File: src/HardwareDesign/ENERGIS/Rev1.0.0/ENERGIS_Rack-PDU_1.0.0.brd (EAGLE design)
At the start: 210 x 108 mm, 395 parts, among them IC1 MP2315GJ-Z, IC10 HLW8032, IC11 HLW8032, IC12 HLW8032, IC13 MP150GJ, IC14 HLW8032, IC15 RP2040, IC16 HLW8032, IC17 MCP6001R, IC18 W25Q128JVPIQ, IC19 CAT24C512HU5IGT3, IC2 MP2315S, IC20 W5500, IC21 MIC5504-3.3YM5-TR, IC22 MCP6001R, IC3 ULN2803A, IC4 MCP23017-E/ML, IC5 MP150GJ, IC6 HLW8032, IC7 HLW8032, IC8 HLW8032, IC9 SN74HC151PWR, J10 0R, J2 JP, J7 JP, J8 0R, J9 0R, K1 G2RL-1A-E_DC12, K2 G2RL-1A-E_DC12, K3 G2RL-1A-E_DC12, K4 G2RL-1A-E_DC12, K5 G2RL-1A-E_DC12, K6 G2RL-1A-E_DC12, K7 G2RL-1A-E_DC12, K8 G2RL-1A-E_DC12, P12ON LEDC1608X35N_FLAT-G, P3ON LEDC1608X35N_FLAT-G, P5ON LEDC1608X35N_FLAT-G, SW3 TP, X1 12MHz, X2 25MHz

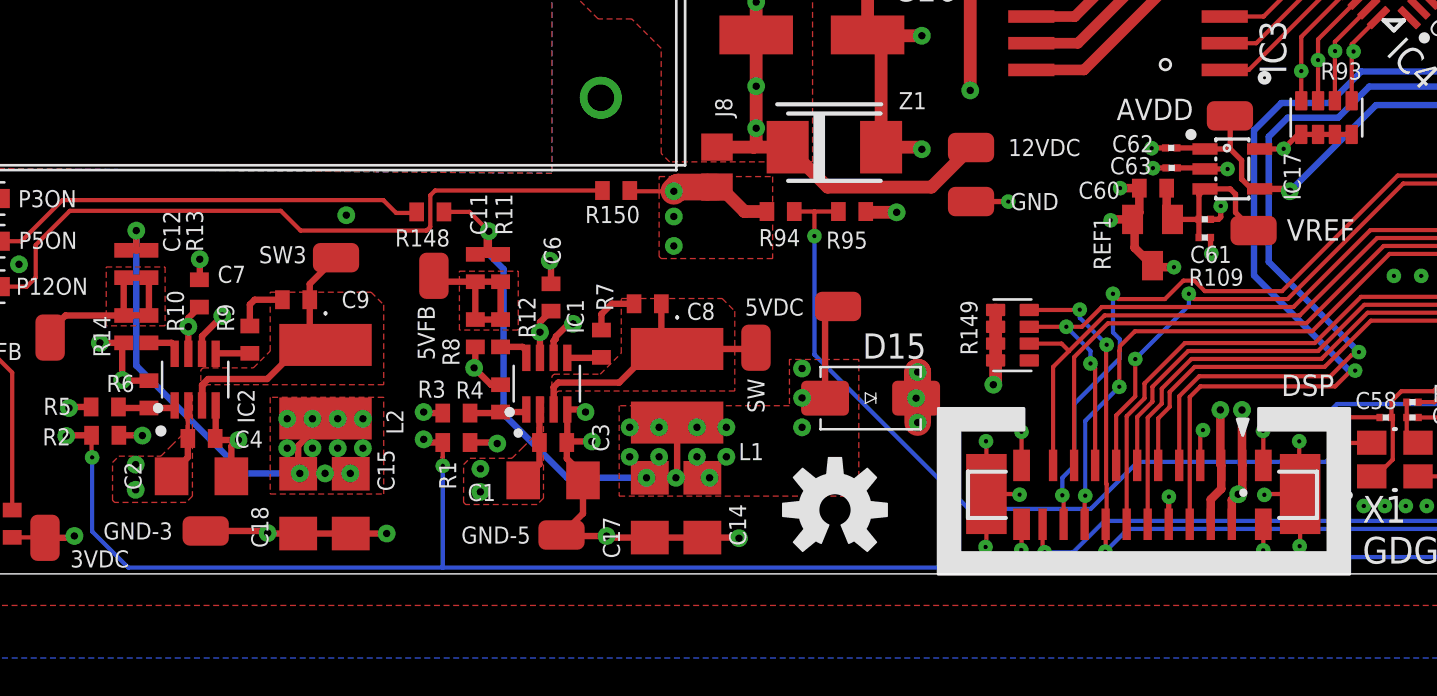
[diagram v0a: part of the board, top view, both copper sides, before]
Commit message: starting with documentation
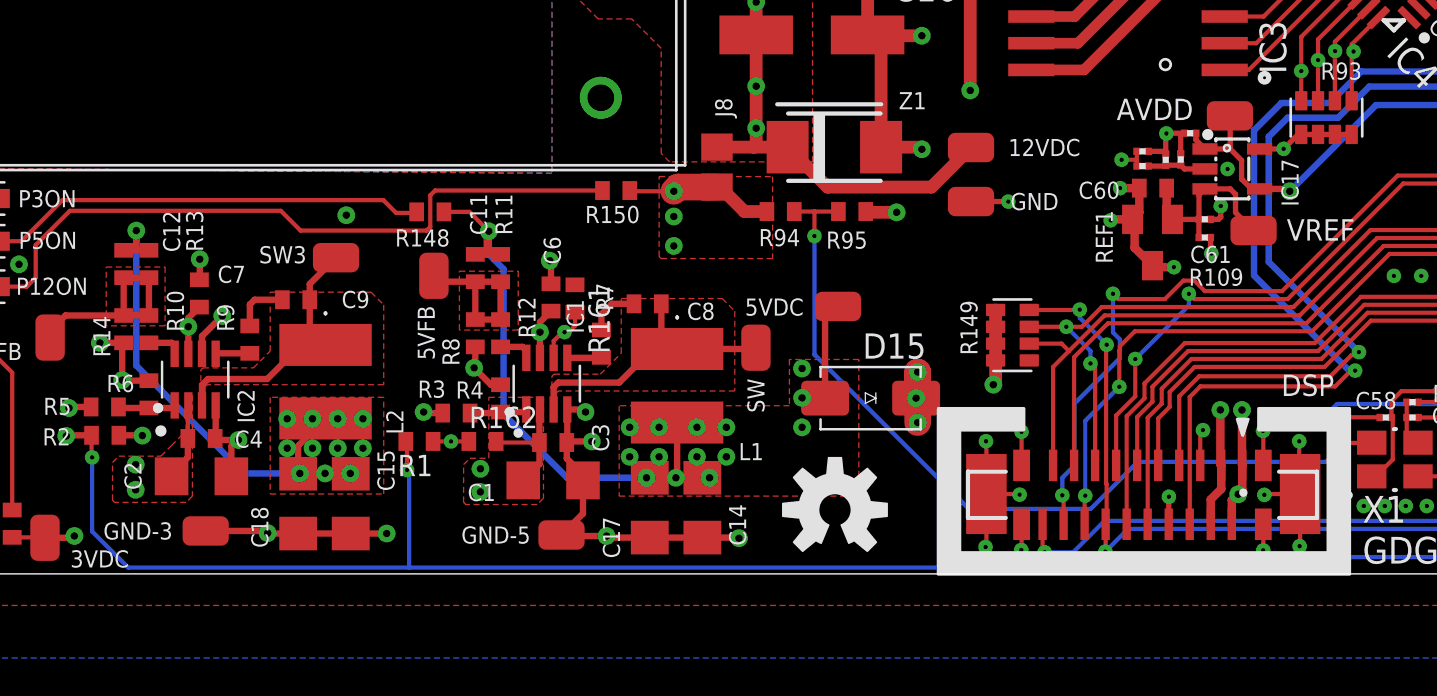
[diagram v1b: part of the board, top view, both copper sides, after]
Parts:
- added C102, C104: 1uF, ds_passive:0201
- added R152: 10R, ds_passive:R0201
- added R161: DNI, ds_passive:0402
- added R162: 10K, ds_passive:0402
- R1: value 10K -> DNI
- moved R1 1.76 mm to (102.1, 6.30)
- moved C62 1.14 mm to (138.8, 21.0)
- moved C63 0.59 mm to (138.3, 19.7), turned to 90 degrees
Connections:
- new net 5V_EN: IC1.6, R1.1, R161.2, R162.1
- new net MCP_VIN: C102.1, C63.1, IC17.2, R152.2
- net +12V: now also R162.2
- net +3V3_MCU: now also C104.1, R152.1; no longer C63.1, IC17.2
- net BUCK_EN: no longer IC1.6
- net GND: now also C102.2, C104.2, R161.1; no longer R1.1
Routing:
- net BUCK_EN: track 135.8 -> 122.3 mm, vias 7 -> 5
- net 5V_EN: track 0.00 -> 13.3 mm, vias 0 -> 2
- net +3V3_MCU: track 114.0 -> 118.3 mm, vias 18 -> 19
- net MCP_VIN: track 0.00 -> 2.78 mm
- net +12V: track 368.3 -> 370.4 mm
- net GND: track 268.2 -> 269.3 mm, vias 172 -> 170
